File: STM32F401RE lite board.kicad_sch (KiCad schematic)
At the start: 45 parts, among them J1 USB_B_Micro, J2 Conn_01x04_Pin, J3 Conn_01x05_Pin, J4 Conn_01x04_Pin, J5 Conn_01x05_Pin, J7 Conn_01x19_Pin, J8 Conn_01x22_Pin, SW1 SW_Push, SW2 SW_SPDT, U1 USBLC6-2SC6, U2 LD3985M33R_SOT23, U3 STM32F401RETx, Y1 8MHz(16pF)

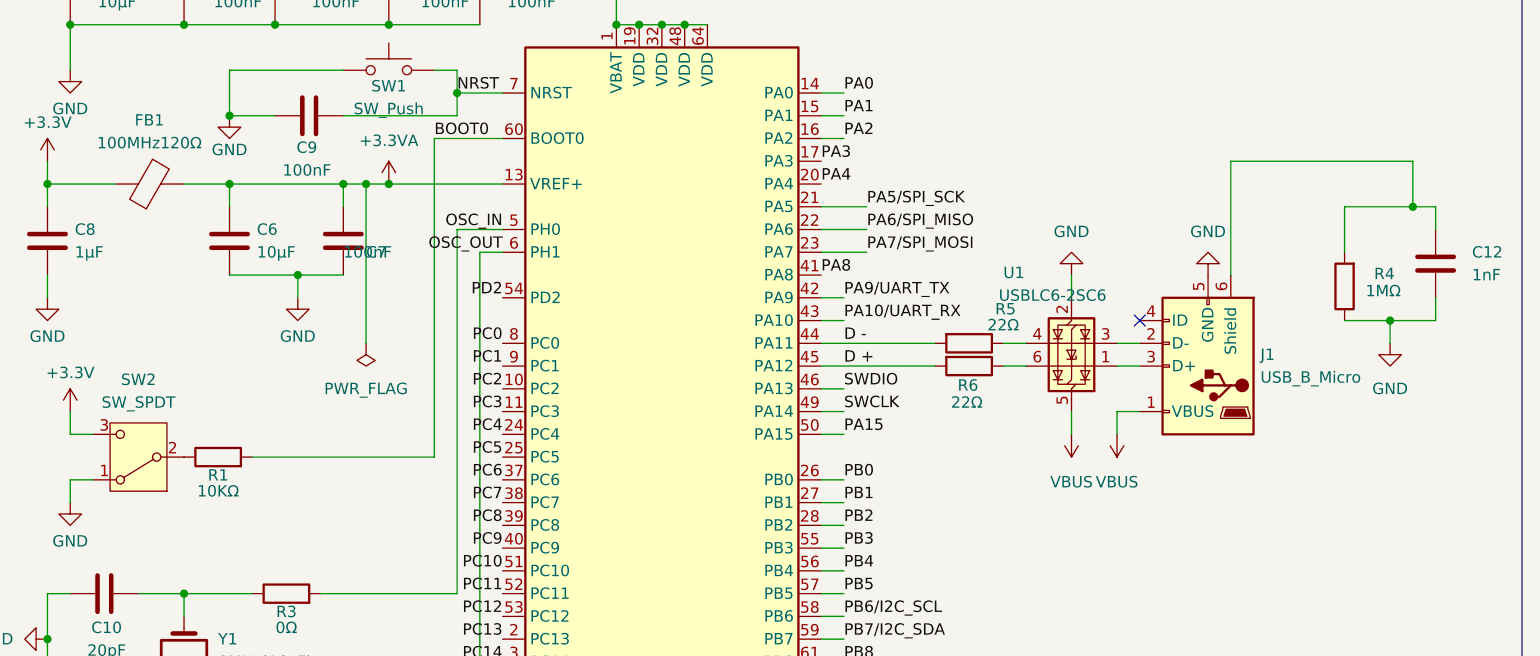
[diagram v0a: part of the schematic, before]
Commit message: C9
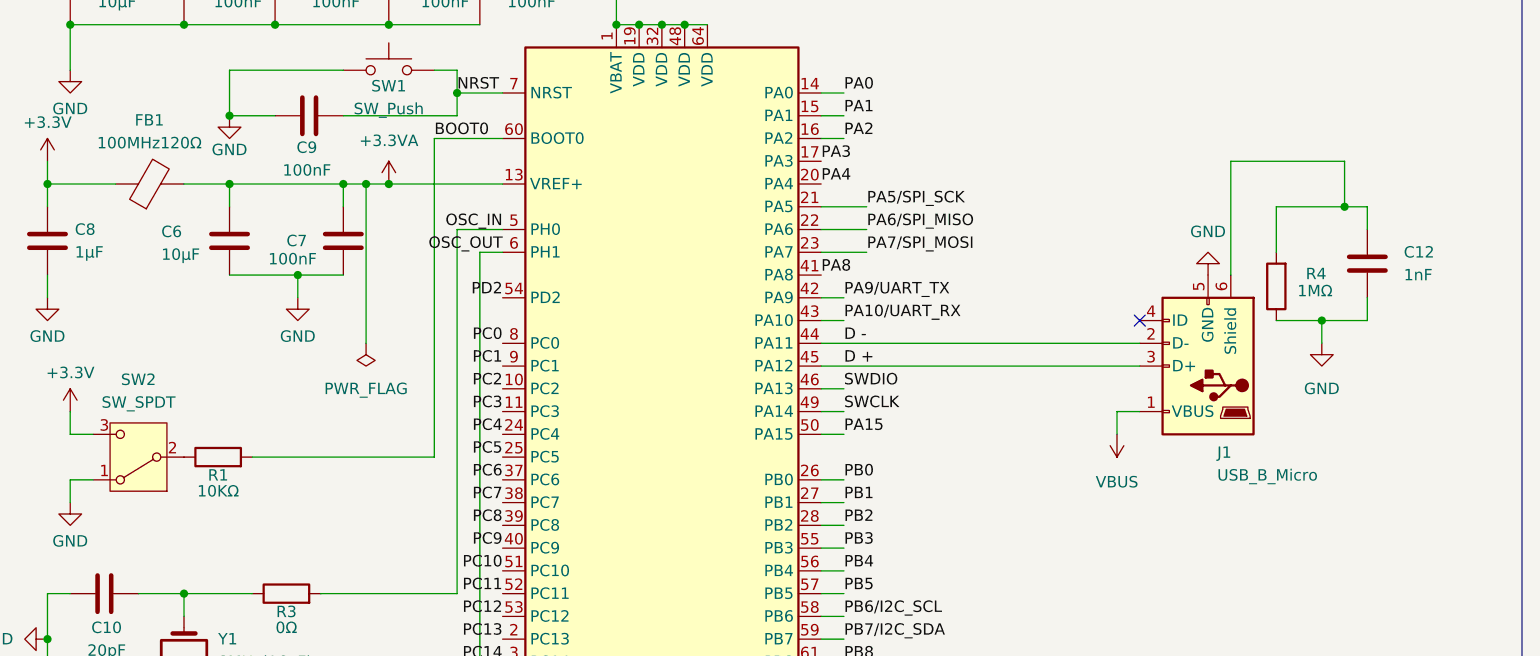
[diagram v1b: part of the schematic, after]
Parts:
- removed R5, R6: 22Ω, Resistor_SMD:R_0402_1005Metric, symbol Device:R
- removed U1: USBLC6-2SC6, Package_TO_SOT_SMD:SOT-23-6, symbol Power_Protection:USBLC6-2SC6
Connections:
- net D +: now also J1.3 (D+)
- net D -: now also J1.2 (D-)
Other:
- moved on the sheet: C12, R4
